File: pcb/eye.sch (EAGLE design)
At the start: 89 parts, among them J2 JST-ZH-5SMD-RA, U1 WS2812, U10 WS2812, U11 WS2812, U12 WS2812, U13 WS2812, U14 WS2812, U15 WS2812, U16 WS2812, U17 WS2812, U18 WS2812, U19 WS2812, U2 WS2812, U20 WS2812, U21 WS2812, U22 WS2812, U23 WS2812, U24 WS2812, U25 WS2812, U26 WS2812, U27 WS2812, U28 WS2812, U29 WS2812, U3 WS2812, U30 WS2812, U31 WS2812, U32 WS2812, U33 WS2812, U34 WS2812, U35 WS2812, U36 WS2812, U37 WS2812, U38 WS2812, U39 WS2812, U4 WS2812, U40 WS2812, U41 WS2812, U42 WS2812, U43 WS2812, U44 WS2812, U45 WS2812, U46 WS2812, U47 WS2812, U48 WS2812, U49 WS2812, U5 WS2812, U50 WS2812, U51 WS2812, U52 WS2812, U53 WS2812, U54 WS2812, U55 WS2812, U56 WS2812, U57 WS2812, U58 WS2812, U59 WS2812, U6 WS2812, U60 WS2812, U61 32U4, U7 WS2812, U8 WS2812, U9 WS2812, X1 ECS-160-20-3X-TR

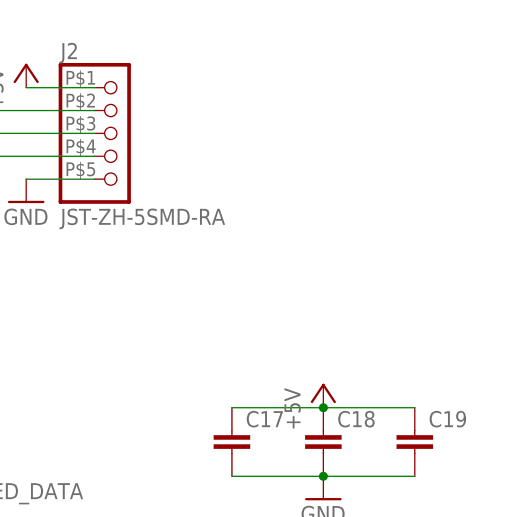
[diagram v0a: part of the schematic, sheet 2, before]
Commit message: optimize some routing
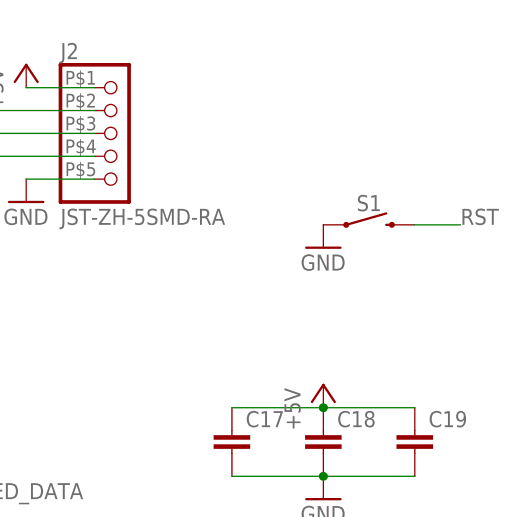
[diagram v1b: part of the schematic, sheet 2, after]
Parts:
- added S1: MOMENTARY-SWITCH-SPST-SMD-6.0X3.5MM, SparkFun-Switches:MOMENTARY-SWITCH-SPST-SMD-6.0X3.5MM
- X1: device SparkFun-Clocks:CRYSTALSMD-3.2X1.5 -> SparkFun-Clocks:CRYSTALSMD-5X3.2-2PAD
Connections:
- net GND: now also S1.1
- net RST: now also S1.2
